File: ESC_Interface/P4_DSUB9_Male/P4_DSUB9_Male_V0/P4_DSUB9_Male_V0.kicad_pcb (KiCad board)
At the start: 2 copper layers, 16.1 x 12 mm, 2 parts, among them J5 Conn_2Rows-09Pins, P4 DE9_Receptacle_MountingHoles

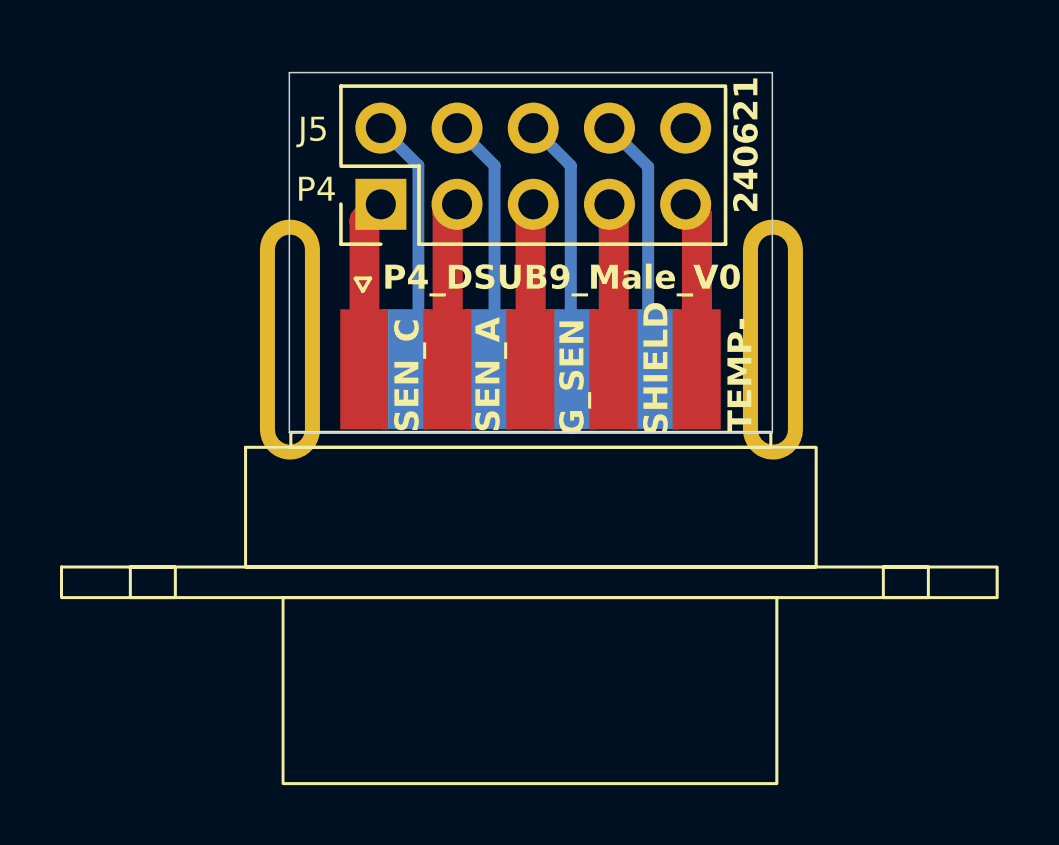
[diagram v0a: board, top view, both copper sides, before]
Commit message: Add files via upload
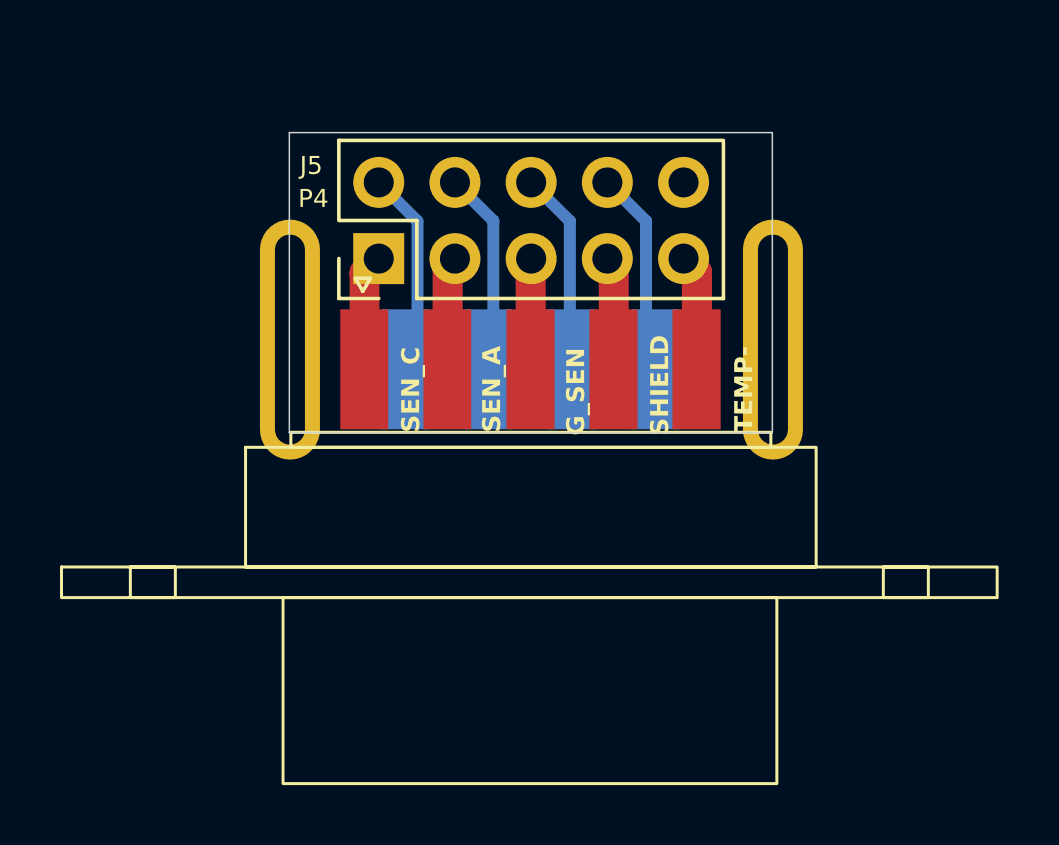
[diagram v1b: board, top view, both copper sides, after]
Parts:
- moved J5 1.81 mm to (133.4, 73.2)
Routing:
- net /SEN_A: track 5.78 -> 3.94 mm
- net /GEN_SEN: track 5.68 -> 3.85 mm
- net /SEN_C: track 5.88 -> 4.04 mm
- net /SEN_B: track 8.88 -> 7.07 mm
- net +12V: track 8.73 -> 6.95 mm
- net /SHIELD: track 5.71 -> 3.93 mm
- net /TEMP+: track 8.82 -> 7.04 mm
- net /TEMP-: track 5.80 -> 4.02 mm
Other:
- board size 16.1 x 12 mm -> 16.1 x 10 mm
